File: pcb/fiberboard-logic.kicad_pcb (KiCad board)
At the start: 2 copper layers, 118 x 84 mm, 81 parts, among them J1 VIN, J2 KB24, J3 FOOT, J4 NPN, J5 RLY1, J6 RLY2, J7 SOL, J8 RS485-2EDG3P, K1 G6KU-2F-Y, K2 G6KU-2F-Y, Q12 AO4407A, Q3 2N3904, Q4 2N3904, Q5 AO3400A, U1 ESP32-DevKitC-32E, U2 XL1509-5.0, U3 AMS1117-3.3, U5 PC817, U6 PC817, U7 MAX485E

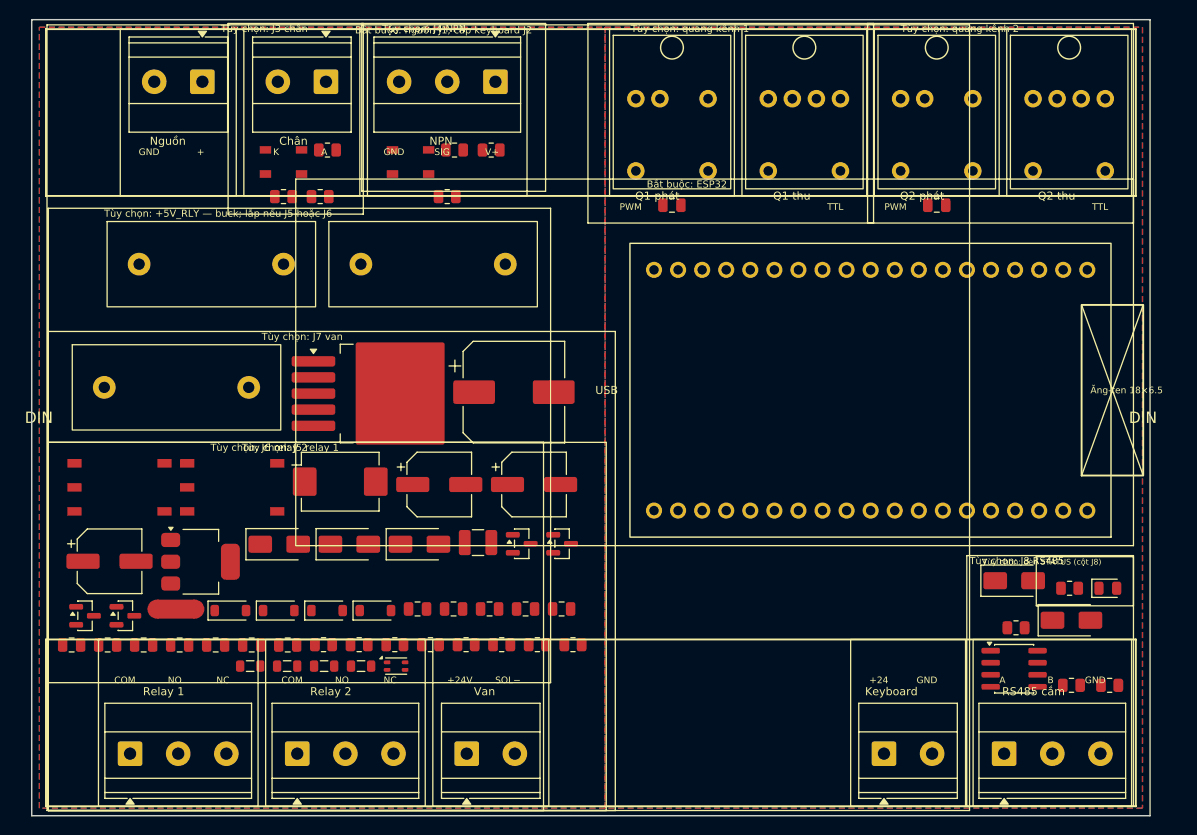
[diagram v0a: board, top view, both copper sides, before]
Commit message: chia vùng linh kiện để sắp xếp và tránh linh kiện quá dày
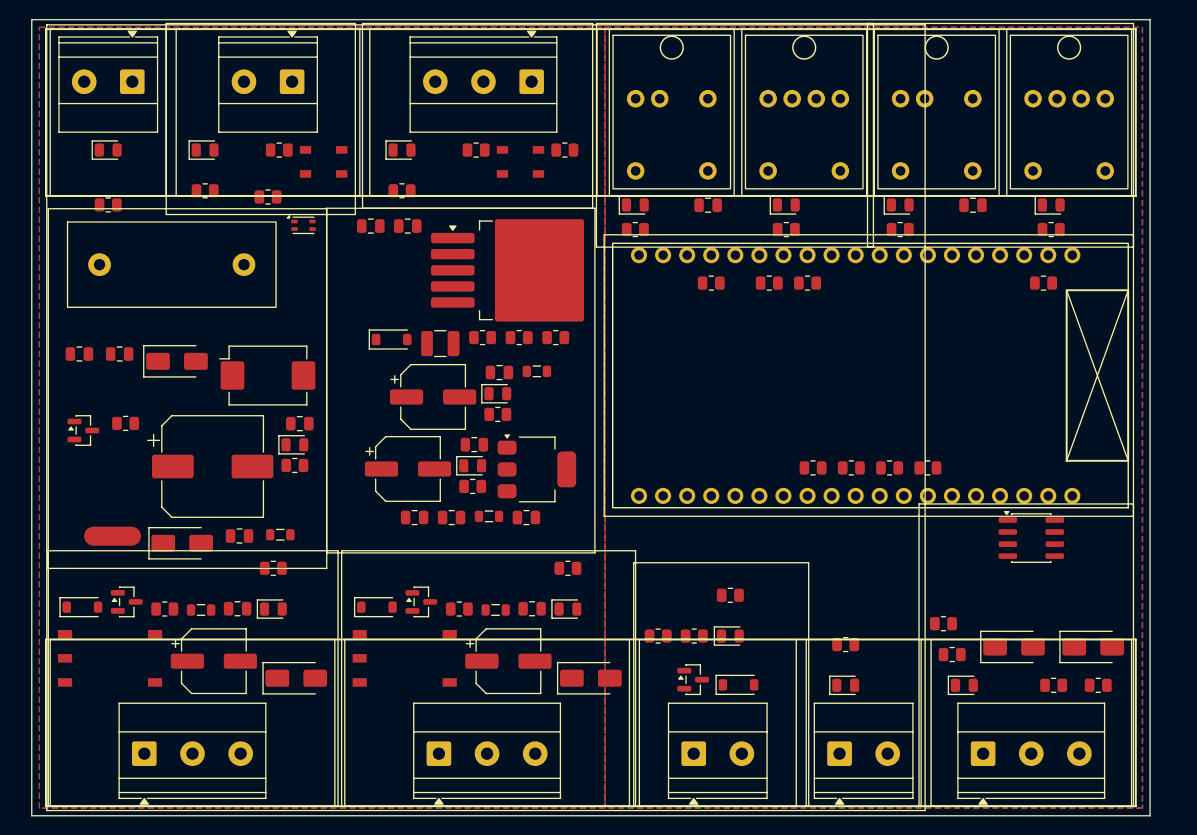
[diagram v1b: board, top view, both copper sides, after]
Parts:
- removed F2: 5x20 F0.5A, Fiberboard:Fuseholder_5x20mm_Horizontal
- removed F3: 5x20 F0.25A, Fiberboard:Fuseholder_5x20mm_Horizontal
- added C26: 220uF, Capacitor_SMD:CP_Elec_6.3x5.4, F.Cu at (50.3, 67.7)
- added C27: 100nF, Capacitor_SMD:C_0805_2012Metric, F.Cu at (52.8, 62.2)
- added D13: VIN, LED_SMD:LED_0805_2012Metric, F.Cu at (8.07, 13.8)
- added D14: KB24, LED_SMD:LED_0805_2012Metric, F.Cu at (85.9, 70.2)
- added D15: FOOT, LED_SMD:LED_0805_2012Metric, F.Cu at (18.3, 13.8)
- added D16: NPN, LED_SMD:LED_0805_2012Metric, F.Cu at (39.1, 13.8)
- added D17: RLY1, LED_SMD:LED_0805_2012Metric, F.Cu at (25.5, 62.2)
- added D18: RLY2, LED_SMD:LED_0805_2012Metric, F.Cu at (56.6, 62.2)
- added D19: VAN, LED_SMD:LED_0805_2012Metric, F.Cu at (73.7, 65.0)
- added D20: 485, LED_SMD:LED_0805_2012Metric, F.Cu at (98.4, 70.2)
- added D21: TX1, LED_SMD:LED_0805_2012Metric, F.Cu at (63.7, 19.6)
- added D22: RX1, LED_SMD:LED_0805_2012Metric, F.Cu at (79.6, 19.6)
- added D23: TX2, LED_SMD:LED_0805_2012Metric, F.Cu at (91.6, 19.6)
- added D24: RX2, LED_SMD:LED_0805_2012Metric, F.Cu at (107.6, 19.6)
- added D25: 5V, LED_SMD:LED_0805_2012Metric, F.Cu at (49.2, 39.5)
- added D26: SMAJ5.0A, Diode_SMD:D_SMA, F.Cu at (59.0, 69.5)
- added D27: 24V, LED_SMD:LED_0805_2012Metric, F.Cu at (27.8, 44.9)
- added FB5: BLM21PG121, Inductor_SMD:L_0805_2012Metric, F.Cu at (48.9, 62.3)
- added R22: 10k, Resistor_SMD:R_0805_2012Metric, F.Cu at (8.07, 19.6)
- added R23: 10k, Resistor_SMD:R_0805_2012Metric, F.Cu at (85.9, 65.9)
- added R24: 1k, Resistor_SMD:R_0805_2012Metric, F.Cu at (18.3, 18.1)
- added R25: 1k, Resistor_SMD:R_0805_2012Metric, F.Cu at (39.1, 18.1)
- added R26: 1k, Resistor_SMD:R_0805_2012Metric, F.Cu at (25.5, 57.9)
- added R27: 1k, Resistor_SMD:R_0805_2012Metric, F.Cu at (56.6, 57.9)
- added R28: 10k, Resistor_SMD:R_0805_2012Metric, F.Cu at (73.7, 60.7)
- added R29: 1k, Resistor_SMD:R_0805_2012Metric, F.Cu at (96.2, 63.7)
- added R30: 1k, Resistor_SMD:R_0805_2012Metric, F.Cu at (63.7, 22.1)
- added R31: 1k, Resistor_SMD:R_0805_2012Metric, F.Cu at (79.6, 22.1)
- added R32: 1k, Resistor_SMD:R_0805_2012Metric, F.Cu at (91.6, 22.1)
- added R33: 1k, Resistor_SMD:R_0805_2012Metric, F.Cu at (107.6, 22.1)
- added R34: 1k, Resistor_SMD:R_0805_2012Metric, F.Cu at (49.2, 41.6)
- added R39: 10k, Resistor_SMD:R_0805_2012Metric, F.Cu at (27.8, 47.0)
- added R40: 1k, Resistor_SMD:R_0805_2012Metric, F.Cu at (94.6, 47.3)
- added R41: 1k, Resistor_SMD:R_0805_2012Metric, F.Cu at (90.5, 47.3)
- added R42: 1k, Resistor_SMD:R_0805_2012Metric, F.Cu at (77.8, 27.8)
- added R43: 1k, Resistor_SMD:R_0805_2012Metric, F.Cu at (71.7, 27.8)
- added R44: 1k, Resistor_SMD:R_0805_2012Metric, F.Cu at (106.8, 27.8)
- added R45: 1k, Resistor_SMD:R_0805_2012Metric, F.Cu at (81.9, 27.8)
- D6: value STATUS -> 3V3
- moved D6 68.2 mm to (46.5, 47.1)
- moved R16 63.9 mm to (46.5, 49.2)
- moved R20 62.9 mm to (86.5, 47.3)
- moved Q5 60.3 mm to (69.8, 69.6)
- moved C17 56.7 mm to (39.7, 21.8)
- moved R21 48.1 mm to (82.4, 47.3)
- moved Q12 47.8 mm to (5.45, 43.4)
- moved L2 47.5 mm to (28.7, 21.7)
- moved Q3 46.3 mm to (10.0, 61.4)
- moved C16 45.1 mm to (35.8, 21.8)
- moved C19 44.7 mm to (5.03, 35.3)
- moved C15 44.3 mm to (9.28, 35.3)
- moved C5 44.3 mm to (49.4, 37.2)
- moved C7 44.1 mm to (46.7, 44.8)
- moved FB2 40.8 mm to (53.3, 37.1)
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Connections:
- net FOOT_LED renamed FOOT_AN
- net NPN_LED renamed NPN_AN
- net STAT_LED renamed P3V3_AN
- C24 pad 1: +5V_RLY -> +5V_RLY1
- C25 pad 1: +5V_RLY -> +5V_RLY1
- D12 pad 1: +5V_RLY -> +5V_RLY1
- D3 pad 1: +5V_RLY -> +5V_RLY1
- D4 pad 1: +5V_RLY -> +5V_RLY2
- D5 pad 1: +24V_SOL -> +24V
- F1R pad 1: FIBER1_DIG -> FIBER1_RX
- F1T pad 4: FIBER1_PWM -> FIBER1_TX
- F2R pad 1: FIBER2_DIG -> FIBER2_RX
- F2T pad 4: FIBER2_PWM -> FIBER2_TX
- FB4 pad 2: +5V_RLY -> +5V_RLY1
- J7 pad 1: +24V_SOL -> +24V
- K1 pad 1: +5V_RLY -> +5V_RLY1
- K2 pad 1: +5V_RLY -> +5V_RLY2
- U7 pad 1: RS485_RX -> RS485_RO
- U7 pad 4: RS485_TX -> RS485_DI
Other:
- board text added: "24V"
- board text added: "3V3"
- board text added: "5V"
- board text added: "Bắt buộc: J1 nguồn vào, J2 cấp bàn phím"
- board text added: "Bắt buộc: MCU"
- board text added: "Bắt buộc: buck 5 V / LDO 3,3 V"
- board text added: "Bắt buộc: bảo vệ 24 V"
- board text added: "C 1000uF"
- board text added: "C 100nF"
- board text added: "C 10uF"
- board text added: "C 220uF"
- board text added: "C 22uF"
- board text added: "MOS"
- board text added: "R 100"
- board text added: "R 100k"
- board text added: "R 10R"
- board text added: "R 10k"
- board text added: "R 1k"
- board text added: "R 3k"
- board text removed: "Bắt buộc: ESP32"
- board text removed: "Bắt buộc: nguồn J1, cấp keyboard J2"
- board text removed: "Tùy chọn: +5V_RLY — buck; lắp nếu J5 hoặc J6"
- board text removed: "Tùy chọn: đèn STATUS (cột J8)"
- board text removed: "USB"
- board text removed: "Ăng-ten 18×6.5"
